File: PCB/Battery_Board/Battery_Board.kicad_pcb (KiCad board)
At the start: 2 copper layers, 90 x 90 mm, 4 parts, among them J1 SE2-30

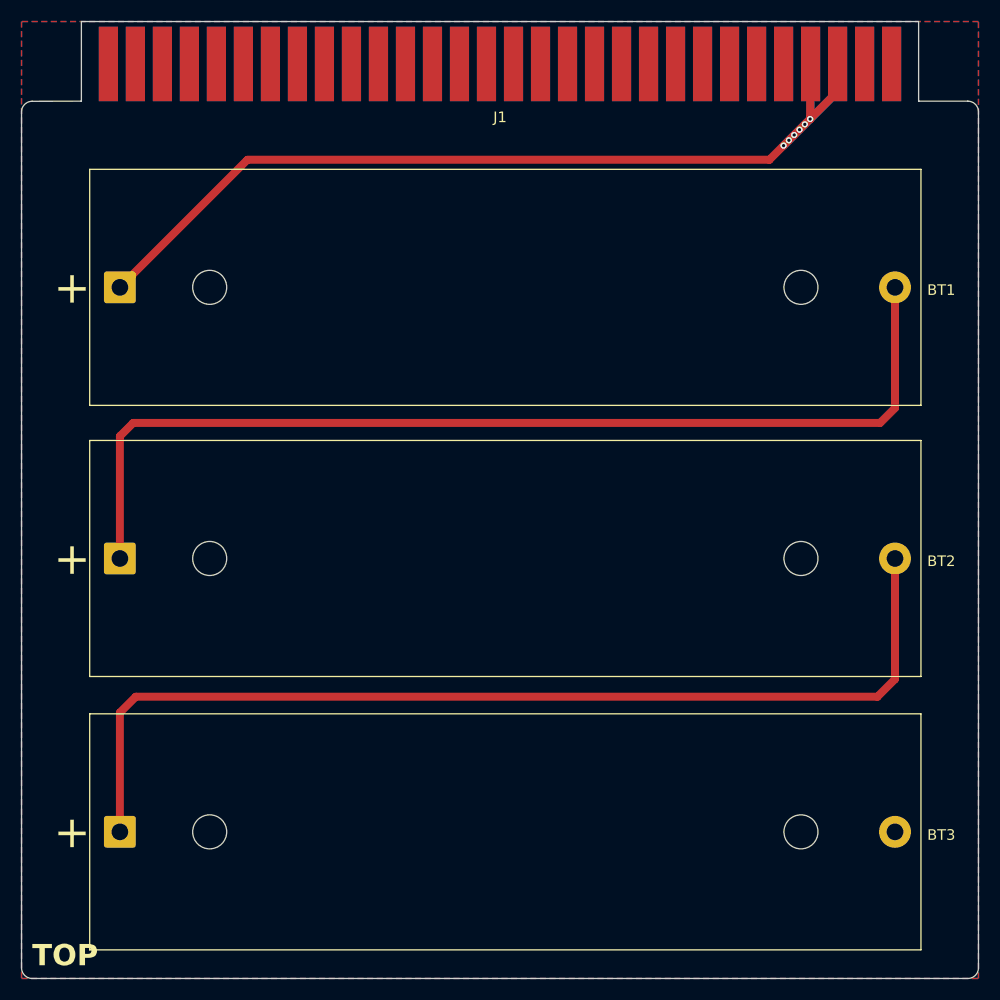
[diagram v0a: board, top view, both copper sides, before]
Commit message: edits from meeting
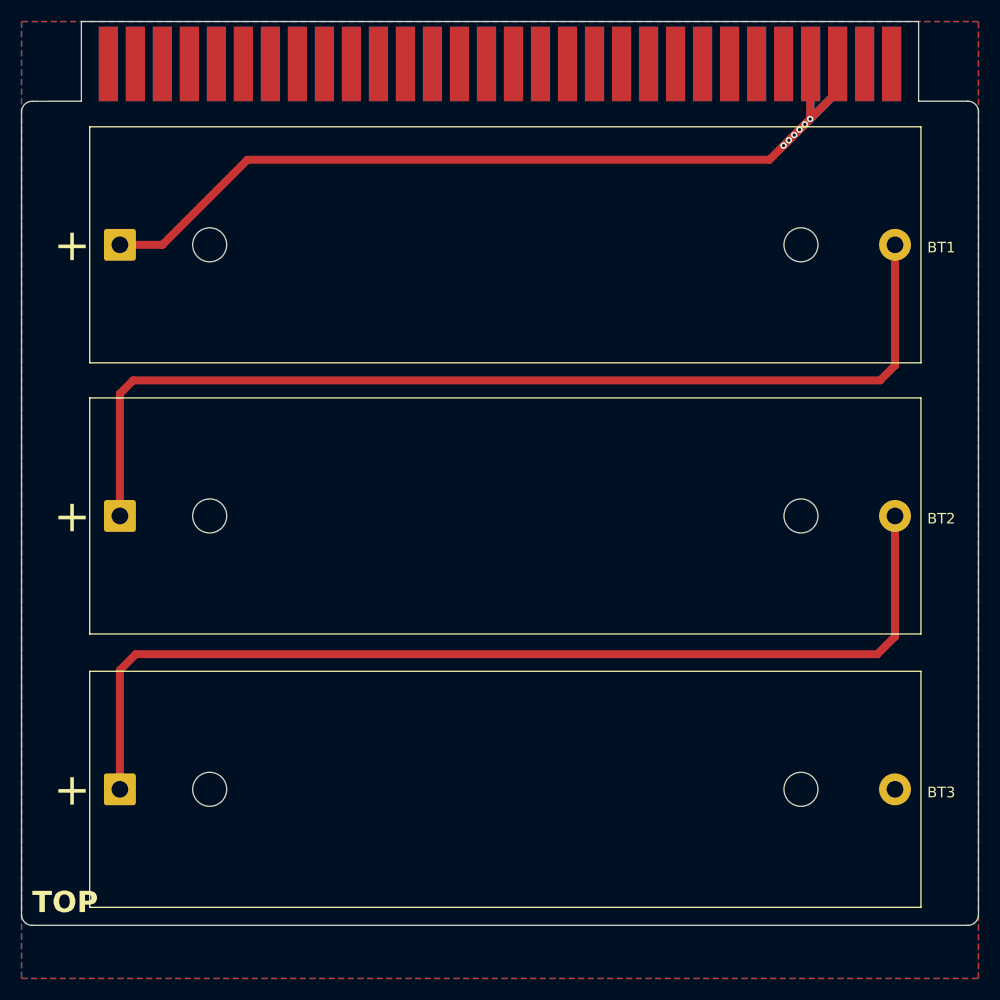
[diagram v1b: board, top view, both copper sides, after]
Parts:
- moved BT1 4.00 mm to (181.8, 63.0)
- moved BT2 4.00 mm to (181.8, 88.5)
- moved BT3 4.00 mm to (181.8, 114.2)
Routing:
- net VBUS: track 97.8 -> 96.2 mm
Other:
- board size 90 x 90 mm -> 90 x 85 mm
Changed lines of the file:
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@@
 			(unlocked yes)
 			(layer "F.SilkS")
+			(hide yes)
 			(effects
 				(font
@@
 		)
 		(fp_line
-			(start -45 4.500001)
-			(end -45 85)
+			(start -45 4.5)
+			(end -45 80.01)
 			(stroke
 				(width 0.05)
-				(type default)
+				(type solid)
 			)
 			(layer "Edge.Cuts")
 		)
 		(fp_line
-			(start -44 86)
-			(end 44 86)
+			(start -44 81)
+			(end 44 81)
 			(stroke
 				(width 0.05)
@@
 		(fp_line
 			(start 45 4.49)
-			(end 45 85)
+			(end 45 80)
 			(stroke
 				(width 0.05)
-				(type default)
+				(type solid)
 			)
 			(layer "Edge.Cuts")
@@
 		)
 		(fp_arc
-			(start -44 86)
-			(mid -44.707107 85.707107)
-			(end -45 85)
+			(start -44 81)
+			(mid -44.707107 80.707107)
+			(end -45 80)
 			(stroke
 				(width 0.05)
@@
 		)
 		(fp_arc
-			(start 45 85)
-			(mid 44.707107 85.707107)
-			(end 44 86)
+			(start 45 80)
+			(mid 44.707107 80.707107)
+			(end 44 81)
 			(stroke
 				(width 0.05)
@@
 		)
 		(fp_text user "TOP"
-			(at -44 85 0)
+			(at -44 80 0)
 			(unlocked yes)
 			(layer "F.SilkS")
@@
 		)
 		(fp_text user "BOTTOM"
-			(at -44 85 0)
+			(at -44 80 0)
 			(unlocked yes)
 			(layer "B.SilkS")
@@
 			(layer "Cmts.User")
 			(pts
+				(xy 178.13 42) (xy 256.87 42)
+			)
+			(height -10.5)
+			(orientation 0)
+			(format
+				(prefix "")
+				(suffix "")
+				(units 3)
+				(units_format 0)
+				(precision 4)
+				(suppress_zeroes yes)
+			)
+			(style
+				(thickness 0.1)
+				(arrow_length 1.27)
+				(text_position_mode 0)
+				(arrow_direction outward)
+				(extension_height 0.58642)
+				(extension_offset 0.5)
+				(keep_text_aligned yes)
+			)
+			(gr_text "78.74"
+				(at 217.5 30.4 0)
+				(layer "Cmts.User")
+				(effects
+					(font
+						(size 1 1)
+						(thickness 0.1)
+					)
+				)
+			)
+		)
+		(dimension
+			(type orthogonal)
+			(layer "Cmts.User")
+			(pts
 				(xy 256.87 42) (xy 256.87 49.49)
 			)
@@
 			(layer "Cmts.User")
 			(pts
-				(xy 172.5 132) (xy 262.5 132)
+				(xy 262.5 127.5) (xy 262.207107 49.5)
 			)
-			(height 12)
-			(orientation 0)
+			(height 11.5)
+			(orientation 1)
 			(format
 				(prefix "")
@@
 				(keep_text_aligned yes)
 			)
-			(gr_text "90"
-				(at 217.5 142.85 0)
+			(gr_text "78"
+				(at 272.85 88.5 90)
 				(layer "Cmts.User")
 				(effects
@@
 			(layer "Cmts.User")
 			(pts
-				(xy 178.13 42) (xy 256.87 42)
+				(xy 267.5 127.5) (xy 267.207107 42)
 			)
-			(height -10.5)
-			(orientation 0)
+			(height 11.5)
+			(orientation 1)
 			(format
 				(prefix "")
@@
 			)
 			(style
-				(thickness 0.1)
+				(thickness 0.05)
 				(arrow_length 1.27)
 				(text_position_mode 0)
@@
 				(keep_text_aligned yes)
 			)
-			(gr_text "78.74"
-				(at 217.5 30.4 0)
+			(gr_text "85.5"
+				(at 277.85 84.75 90)
 				(layer "Cmts.User")
 				(effects
 					(font
 						(size 1 1)
-						(thickness 0.1)
+						(thickness 0.15)
 					)
 				)
@@
 			(layer "Cmts.User")
 			(pts
-				(xy 262.5 132) (xy 262.5 49.49)
+				(xy 172.5 127) (xy 262.5 127)
 			)
-			(height 11.5)
-			(orientation 1)
+			(height 12)
+			(orientation 0)
 			(format
 				(prefix "")
@@
 				(keep_text_aligned yes)
 			)
-			(gr_text "82.51"
-				(at 272.85 90.745 90)
+			(gr_text "90"
+				(at 217.5 137.85 0)
 				(layer "Cmts.User")
 				(effects
@@
 		)
 		(group ""
-			(members "0576a331-9f76-401f-ac96-d302c2b2379b" "099aa479-7b72-4a4c-a769-8518bc94f07f"
-				"1f978678-9fc6-4bec-9ca9-02e1599cec2f" "27cee22b-b478-4347-aa44-11140595800f"
-				"29875613-e73a-495e-9083-c9885d887a25" "2a0c306a-fdfe-43d5-a334-9794d8d520a3"
-				"4700ff43-c1d3-4c62-86c6-1426cdb297bd" "572e2d59-fd76-4914-a222-ecfe9b0544c9"
-				"6bf05120-a336-436d-8543-32eb7675340c" "6d798e41-cb84-4aac-abf0-22e6f1867561"
-				"723e9221-29d5-4341-88ad-08831b8e28a3" "7f71f75a-72a5-4812-b113-32c8ab858674"
-				"833661ed-15f4-4b34-b7ac-0dae79ed6555" "886374e7-eb69-42c8-bf5a-29edd44aea2c"
-				"8c5bcbdd-1bc6-4fa8-9cfd-8305585a3a0f" "8ede6605-373b-4457-8394-add15065966f"
-				"8f926001-9687-45b1-af0e-f0e6804b1232" "9616212e-ddeb-464e-ba2a-f3652c605924"
-				"a6f6ed38-8c80-45d3-b3c7-c804da35cb93" "a7b35c75-fda6-4a59-b0b7-3dbb266fe900"
-				"adab6477-f7f5-4164-8f7b-e38af7eb5a59" "b5f7db92-ed44-4e38-bdac-5c0cba2ea7c7"
-				"ce6bccaa-8fed-41bf-aac4-a5a355f3a8b7" "d0f0d393-7671-4937-bf78-a173aa1db914"
-				"dc6bacf0-e5fd-4b17-ae37-7d0142fdcd1c" "dfc64a73-e850-4149-a8c4-79cb9051a176"
-				"e6e6bbec-4fa2-47b2-8fb0-a771e8328cb0" "e8f1f9bd-b0bc-410a-b6fe-93093eb8addd"
-				"f3149af5-1fe6-4d6f-bb96-aaf2cd4da463" "f68173f6-cd59-4c9e-98bc-a7722907d220"
-				"f922a95d-d4cd-4958-ba62-2a210f3c6677"
+			(members "01ceb4d7-95a9-4715-8b54-7b6caa1cadf4" "02076a63-9917-4e24-a663-0149b9bb5b17"
+				"02e9ad1f-8e94-436c-a87a-4f6fb173b84c" "08a04171-eadc-4275-aa42-c85b388e8773"
+				"110bedc4-5d3d-4ae5-b3bc-c95eb5f47476" "1802cfd3-1e43-46db-acbb-099de4b3b90c"
+				"2227c4c2-d2ef-4f95-b9f6-790a28e5d98c" "2abe32f9-517c-4c12-a889-542dc000e172"
+				"2cb27459-94ce-4522-972a-630bd1ebb40d" "38a1d972-df17-4b4f-a38d-c216954af38a"
+				"46406e21-b3fa-4dd2-8b17-17e968e4e5c5" "5ca96600-b42e-42dd-b97f-97355b204386"
+				"65c7c494-3c50-48c8-92cb-db0b18618085" "6c723505-714b-4f0f-a105-da710104e54f"
+				"70d2f12b-4495-4352-873b-5883c26ae163" "7a911669-cc2a-41d0-99fd-a1e85cbb01c7"
+				"7c43dd13-a671-45a3-9476-cfae4376c597" "891dffce-6605-4464-98c8-2f31cfdd79fd"
+				"89aada95-2ee9-4c5b-9339-a7812df6a316" "940b537b-df54-4350-bb10-e3a75d4bcdd0"
+				"9a8d925c-1dfc-47a4-873d-8d99bf2f9ae6" "9d6a41c1-f18f-436b-833d-b316eedfdd30"
+				"9d96d457-b2b6-47cc-a804-3e302d1c7f6d" "ae9afbf3-05ef-4faf-96bb-8ff14be817ec"
+				"be1c2783-6d61-4ae9-bac6-a30863c695ad" "bea0b7e5-06eb-4680-ae37-578f333a01d8"
+				"c8f57011-5123-477d-ae20-199cb2d90c9f" "d5551b4f-07b9-49e6-ac4c-95ea77f40f64"
+				"f1743469-f647-49cf-8a1c-7979b37cce3b" "f184c074-2fca-4ee6-b85a-682eb8421d94"
+				"fae93057-a3b3-4aa7-93e1-f8272b9e41f8"
 			)
 		)
 		(group ""
-			(members "05cd00b3-f595-4347-87c7-70b54c5663ee" "07c7a2e0-46ce-4c1c-90d0-b701c67f37f3"
-				"0e79a1ce-c1ad-4d48-8972-d496fbdfae5b" "1a5604f0-b87b-42cb-83b4-87db2195a045"
-				"212fc3bd-7cea-4ebc-a4ae-d3dc07d95503" "cec5d429-1663-4ff6-ae85-c53572afcdeb"
+			(members "05571765-961c-47ef-875d-9e8820501feb" "0923ca63-275c-462e-ae7b-37d8e9938db9"
+				"2d3d227e-22c0-4674-99fb-4ce77206abb8" "3299c99c-c4bb-4d60-9ffd-9c8dc9cd9578"
+				"6b79917f-da90-47f8-860a-b910efcf7c59" "8acd7ca3-e90a-4b1c-82ba-3497edefcdd9"
 			)
 		)
@@
 	(footprint "Battery:BatteryHolder_MPD_BK-18650-PC2"
 		(layer "F.Cu")
-		(at 181.751029 92.5)
+		(at 181.751029 88.5)
 		(descr "Battery holder, MPD BK-18650, battery type 1x18650, https://www.batteryholders.com/uploads/parts/BK-18650-PC2/datasheets/BK-18650-PC2-datasheet.pdf, generated with kicad-footprint-generator StandardBox_generator.py")
 		(tags "horizontal single")
@@
 	(footprint "Battery:BatteryHolder_MPD_BK-18650-PC2"
 		(layer "F.Cu")
-		(at 181.751029 67)
+		(at 181.751029 63)
 		(descr "Battery holder, MPD BK-18650, battery type 1x18650, https://www.batteryholders.com/uploads/parts/BK-18650-PC2/datasheets/BK-18650-PC2-datasheet.pdf, generated with kicad-footprint-generator StandardBox_generator.py")
 		(tags "horizontal single")
@@
 	(footprint "Battery:BatteryHolder_MPD_BK-18650-PC2"
 		(layer "F.Cu")
-		(at 181.751029 118.21)
+		(at 181.751029 114.21)
 		(descr "Battery holder, MPD BK-18650, battery type 1x18650, https://www.batteryholders.com/uploads/parts/BK-18650-PC2/datasheets/BK-18650-PC2-datasheet.pdf, generated with kicad-footprint-generator StandardBox_generator.py")
 		(tags "horizontal single")
@@
 	)
 	(segment
+		(start 185.751029 63)
+		(end 181.751029 63)
+		(width 0.75)
+		(layer "F.Cu")
+		(net 1)
+	)
+	(segment
 		(start 246.17 51.67)
 		(end 246.67 51.17)
@@
 	)
 	(segment
-		(start 181.751029 67)
-		(end 193.751029 55)
+		(start 244.67 53.17)
+		(end 245.17 52.67)
 		(width 0.75)
 		(layer "F.Cu")
@@
 	)
 	(segment
-		(start 244.67 53.17)
-		(end 245.17 52.67)
+		(start 193.751029 55)
+		(end 185.751029 63)
 		(width 0.75)
 		(layer "F.Cu")
@@
 	)
 	(segment
-		(start 253.251029 79.75)
-		(end 183.001029 79.75)
+		(start 253.251029 75.75)
+		(end 183.001029 75.75)
 		(width 0.75)
 		(layer "F.Cu")
@@
 	)
 	(segment
-		(start 254.651029 78.35)
-		(end 253.251029 79.75)
+		(start 254.651029 74.35)
+		(end 253.251029 75.75)
 		(width 0.75)
 		(layer "F.Cu")
@@
 	)
 	(segment
-		(start 181.751029 81)
-		(end 181.751029 92.5)
+		(start 181.751029 77)
+		(end 181.751029 88.5)
 		(width 0.75)
 		(layer "F.Cu")
@@
 	)
 	(segment
-		(start 254.651029 67)
-		(end 254.651029 78.35)
+		(start 254.651029 63)
+		(end 254.651029 74.35)
 		(width 0.75)
 		(layer "F.Cu")
@@
 	)
 	(segment
-		(start 183.001029 79.75)
-		(end 181.751029 81)
+		(start 183.001029 75.75)
+		(end 181.751029 77)
 		(width 0.75)
 		(layer "F.Cu")
@@
 	)
 	(segment
-		(start 254.651029 92.5)
-		(end 254.651029 103.85)
+		(start 254.651029 88.5)
+		(end 254.651029 99.85)
 		(width 0.75)
 		(layer "F.Cu")
@@
 	)
 	(segment
-		(start 181.751029 107)
-		(end 181.751029 118.21)
+		(start 181.751029 103)
+		(end 181.751029 114.21)
 		(width 0.75)
 		(layer "F.Cu")
@@
 	)
 	(segment
-		(start 253.001029 105.5)
-		(end 183.251029 105.5)
+		(start 253.001029 101.5)
+		(end 183.251029 101.5)
 		(width 0.75)
 		(layer "F.Cu")
@@
 	)
 	(segment
-		(start 183.251029 105.5)
-		(end 181.751029 107)
+		(start 183.251029 101.5)
+		(end 181.751029 103)
 		(width 0.75)
 		(layer "F.Cu")
@@
 	)
 	(segment
-		(start 254.651029 103.85)
-		(end 253.001029 105.5)
+		(start 254.651029 99.85)
+		(end 253.001029 101.5)
 		(width 0.75)
 		(layer "F.Cu")
